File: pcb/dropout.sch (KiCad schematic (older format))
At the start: 64 parts, among them J1 Conn_01x04_Male, SW1 Rotary_Encoder_Switch, SW2 SW_Push, U1 ProMicro, U2 ProMicro

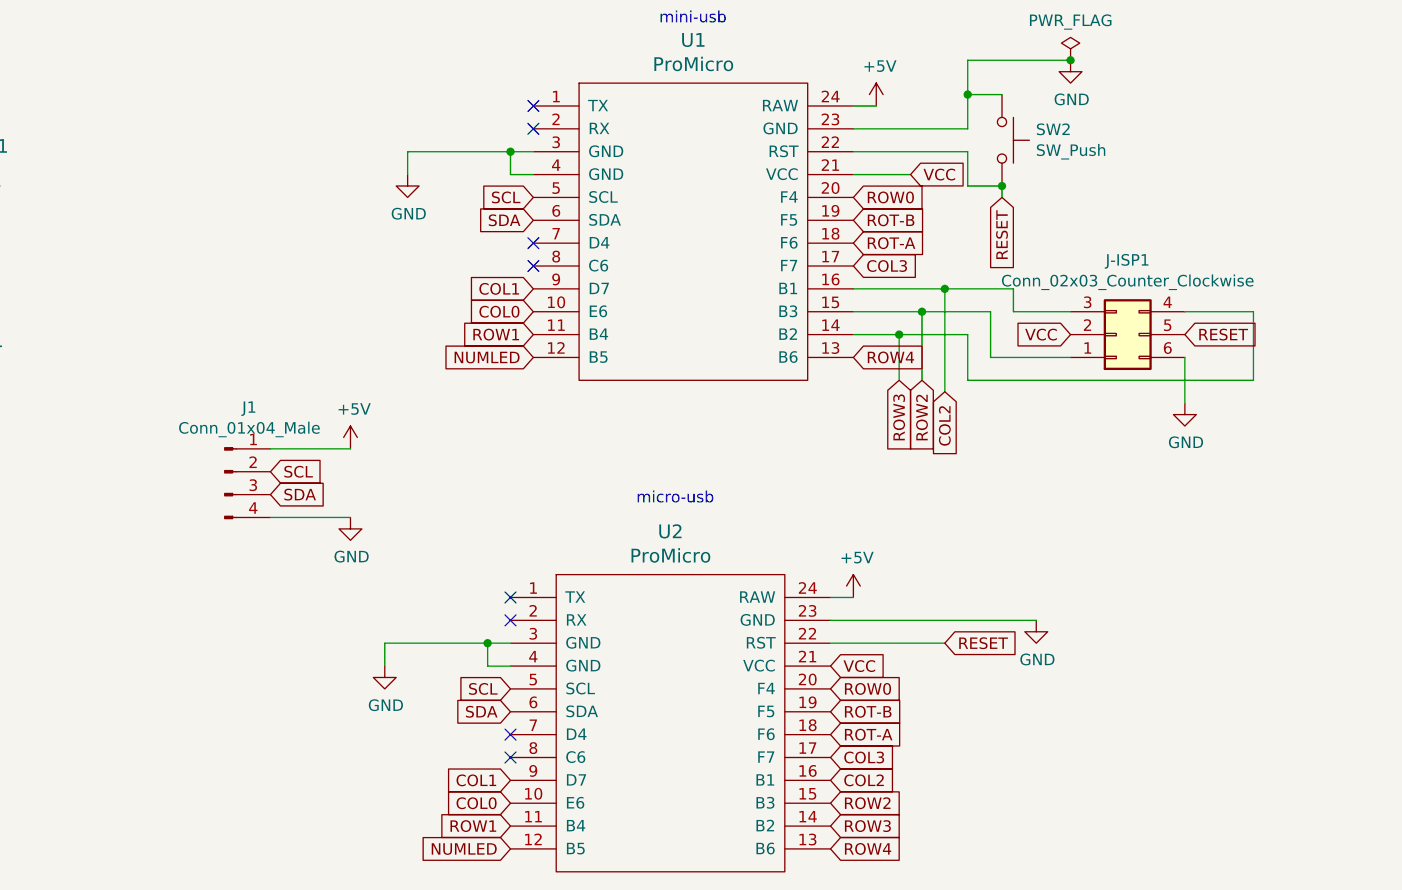
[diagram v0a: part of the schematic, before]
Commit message: updating to rev0.5
updating to rev0.5
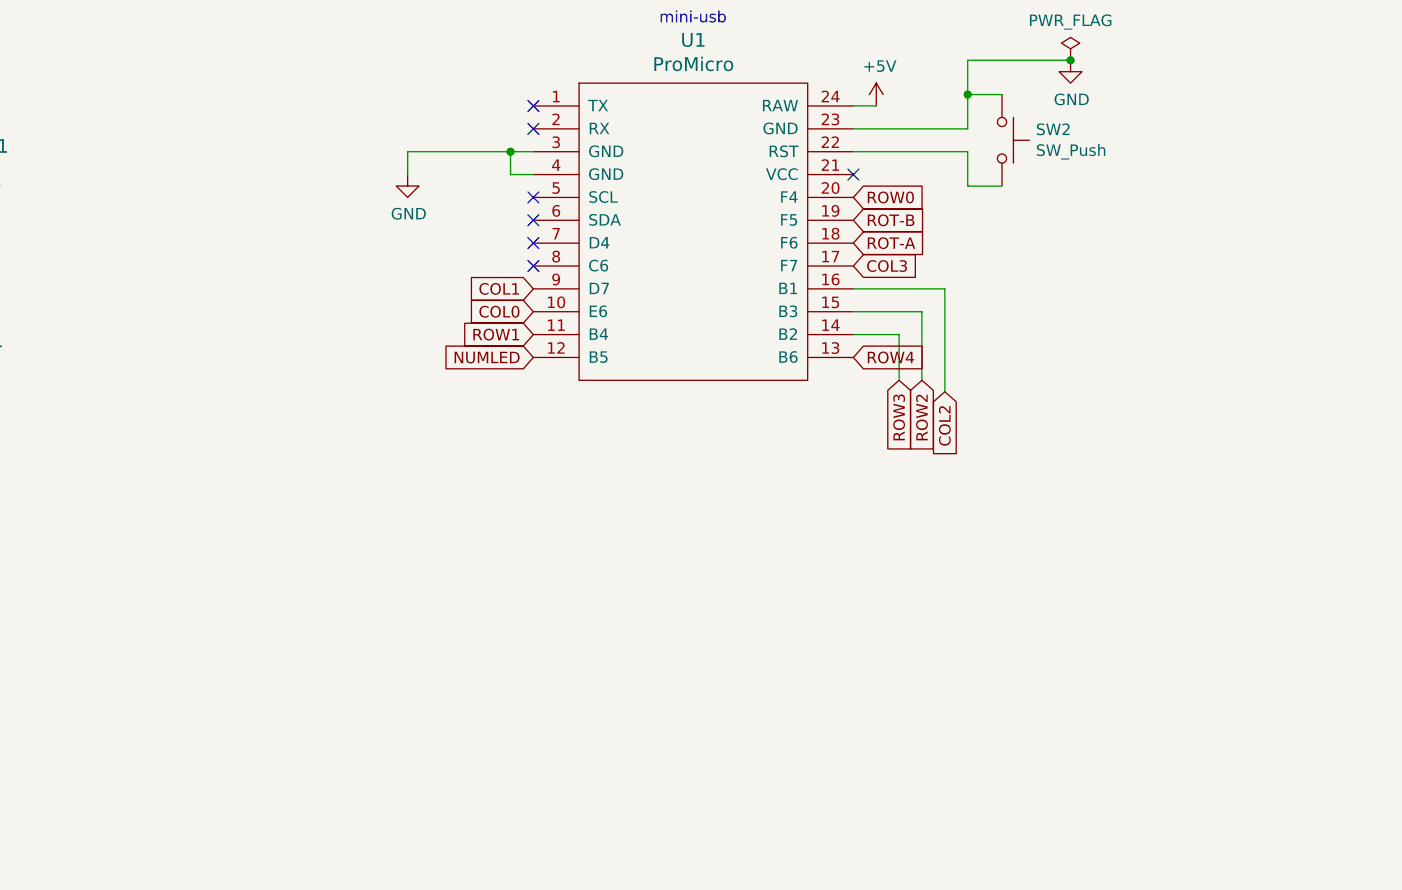
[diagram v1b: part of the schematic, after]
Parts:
- removed J-ISP1: Conn_02x03_Counter_Clockwise, Connector_PinHeader_2.54mm:PinHeader_2x03_P2.54mm_Vertical, symbol Connector_Generic:Conn_02x03_Counter_Clockwise
- removed J1: Conn_01x04_Male, Connector_PinHeader_2.54mm:PinHeader_1x04_P2.54mm_Vertical, symbol Connector:Conn_01x04_Male
- removed U2: ProMicro, Keebio-Parts:ArduinoProMicro, symbol promicro:ProMicro
- D1, D10, D11, D12, D13, D14, D15, D16, D17, D18, D2, D3, D4, D5, D6, D7, D8, D9: footprint Diode_SMD:D_SOD-123 -> footprint:Diode_TH_SOD123
- H16, H17, H18, H19: footprint Panelization:mouse-bite-2mm-slot -> Keebio-Parts:breakaway-mousebites
- K-0, K-ENT1: footprint MX_Only:MXOnly-2U-ReversedStabilizers -> MX_Only:MXOnly-2U-ReversedStabilizers-NoLED
- U1: footprint Keebio-Parts:ArduinoProMicro-Mini-USB -> promicro:ProMico_mini&micro
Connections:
- net RESET: no longer names the net of SW2.2, U1.22 (RST)
- net SCL: no longer names the net of U1.5 (SCL)
- net SDA: no longer names the net of U1.6 (SDA)
- net VCC: no longer names the net of U1.21 (VCC)
- no-connect marks 8 -> 7
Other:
- note removed: "micro-usb\n"
